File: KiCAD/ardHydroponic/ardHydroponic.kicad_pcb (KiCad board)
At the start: 2 copper layers, 7 parts, among them J1 3-pin_IRF5320_MOSFET_module_h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, J2 3-pin_IRF5320_MOSFET_module_h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, J3 3-pin_IRF5320_MOSFET_module_h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, J4 3-pin_IRF5320_MOSFET_module_h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, J5 4-pin_I2C_LCD_header, U1 DS18B20

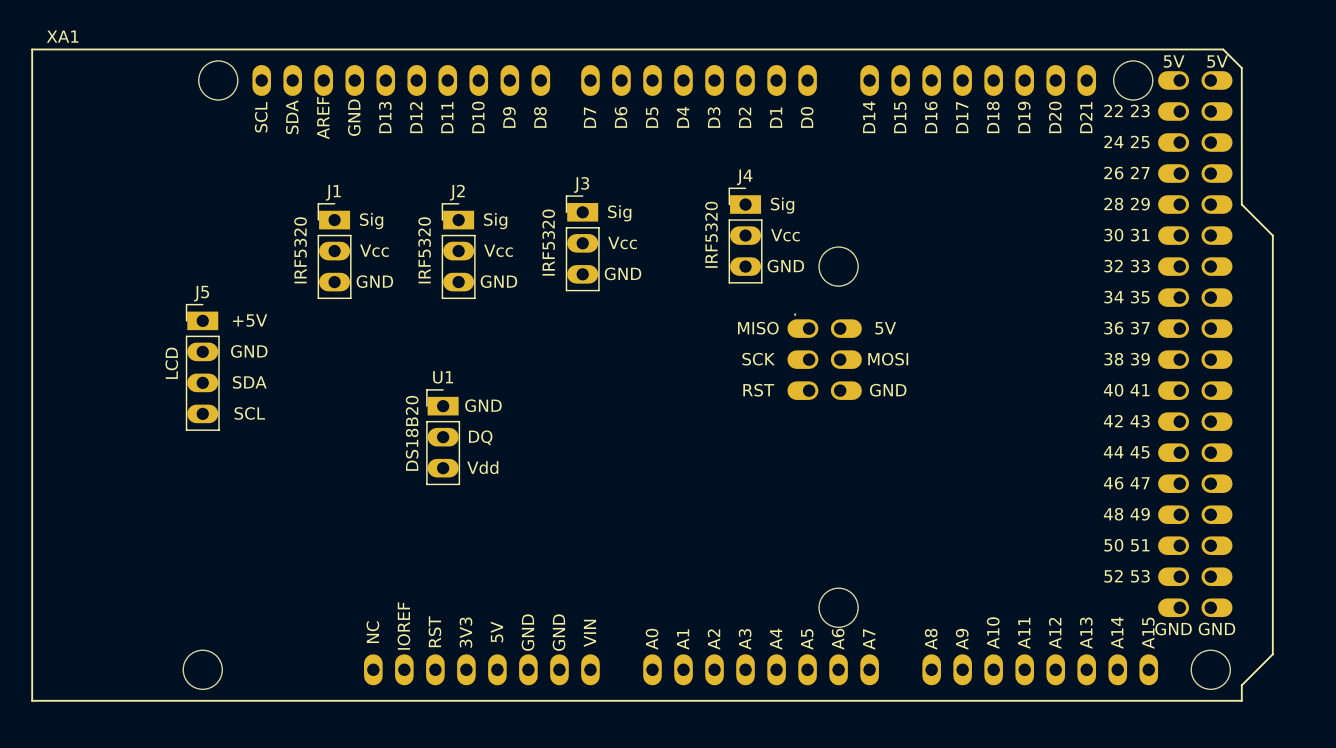
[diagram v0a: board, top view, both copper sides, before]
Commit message: new pins, schematics
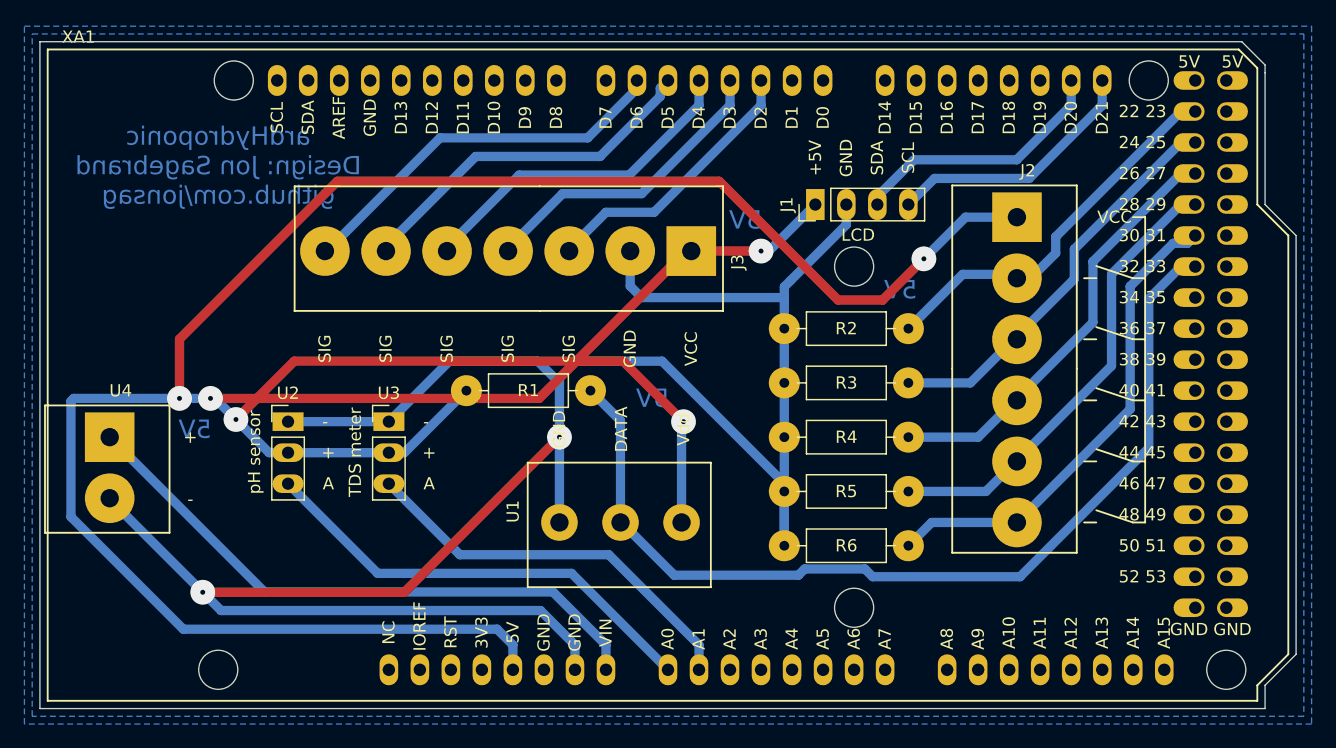
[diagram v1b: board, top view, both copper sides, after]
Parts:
- removed J4: 3-pin_IRF5320_MOSFET_module_header, My_Headers:3-pin_IRF5320_MOSFET_module_header_large
- removed J5: 4-pin_I2C_LCD_header, My_Headers:4-pin_I2C_LCD_header_larger
- added R1: 4.7k, My_Misc:R_Axial_DIN0207_L6.3mm_D2.5mm_P10.16mm_Horizontal_larger_pads, F.Cu at (134.6, 99.1)
- added R2: 10k, My_Misc:R_Axial_DIN0207_L6.3mm_D2.5mm_P10.16mm_Horizontal_larger_pads, F.Cu at (160.7, 94.0)
- added R3: 10k, My_Misc:R_Axial_DIN0207_L6.3mm_D2.5mm_P10.16mm_Horizontal_larger_pads, F.Cu at (160.7, 98.4)
- added R4: 10k, My_Misc:R_Axial_DIN0207_L6.3mm_D2.5mm_P10.16mm_Horizontal_larger_pads, F.Cu at (160.7, 102.9)
- added R5: 10k, My_Misc:R_Axial_DIN0207_L6.3mm_D2.5mm_P10.16mm_Horizontal_larger_pads, F.Cu at (160.7, 107.3)
- added R6: 10k, My_Misc:R_Axial_DIN0207_L6.3mm_D2.5mm_P10.16mm_Horizontal_larger_pads, F.Cu at (160.7, 111.8)
- added U2: pH sensor, My_Headers:3-pin_DFRobot_Gravity_pH-sensor_header_large, F.Cu at (120.0, 101.6)
- added U3: TDS meter, My_Headers:3-pin_DFRobot_Gravity_TDS-meter_header_large, F.Cu at (128.3, 101.6)
- added U4: Power in, My_Parts:2-pole_power_in_screw_terminal, F.Cu at (105.4, 102.9)
- J1: value 3-pin_IRF5320_MOSFET_module_header -> LCD display; footprint My_Headers:3-pin_IRF5320_MOSFET_module_header_large -> My_Headers:4-pin_I2C_LCD_header_larger
- J2: value 3-pin_IRF5320_MOSFET_module_header -> Buttons; footprint My_Headers:3-pin_IRF5320_MOSFET_module_header_large -> My_Parts:6-pole_5-NO_switch_screw_terminal
- J3: value 3-pin_IRF5320_MOSFET_module_header -> MOSFETs; footprint My_Headers:3-pin_IRF5320_MOSFET_module_header_large -> My_Parts:7-pole_6-MOSFET_screw_terminal
- U1: footprint My_Headers:3_pin_Dallas_1-wire_header_larger_pads -> My_Parts:3-pole_DS18B20_screw_terminal
- XA1: footprint My_Arduino:Arduino_Mega2560_Shield_large -> My_Arduino:Arduino_Mega2560_Shield__no_ICSP_large
- moved J2 45.7 mm to (179.7, 84.9)
- moved J1 39.4 mm to (163.2, 83.8), turned to 90 degrees
- moved U1 13.5 mm to (142.2, 109.9), turned to 90 degrees
- moved J3 9.44 mm to (153.0, 87.6), turned to 270 degrees
- moved XA1 1.27 mm to (100.3, 124.5)
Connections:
- J1 pad 1: Net-(J1-Pad1) -> +5V
- J1 pad 3: Net-(J1-Pad3) -> GND
- J2 pad 1: Net-(J2-Pad1) -> +5V
- J2 pad 2: Net-(J2-Pad2) -> button1
- J2 pad 3: Net-(J2-Pad3) -> button2
- J3 pad 1: Net-(J3-Pad1) -> +5V
- J3 pad 2: Net-(J3-Pad2) -> GND
- J3 pad 3: Net-(J3-Pad3) -> pH+
- U1 pad 1: Net-(U1-Pad1) -> GND
- U1 pad 2: Net-(U1-Pad2) -> dallas
- U1 pad 3: Net-(U1-Pad3) -> +5V
- XA1 pad 1: Net-(XA1-Pad1) -> nutrA
- XA1 pad 10: Net-(XA1-Pad10) -> +5V
- XA1 pad 100: Net-(XA1-Pad100) -> +6V
- XA1 pad 15: Net-(XA1-Pad15) -> stirrer
- XA1 pad 43: Net-(XA1-Pad43) -> Net-(J1-Pad7)
- XA1 pad 44: Net-(XA1-Pad44) -> Net-(J1-Pad5)
- XA1 pad 5: Net-(XA1-Pad5) -> nutrB
- XA1 pad 58: Net-(XA1-Pad58) -> dallas
- XA1 pad 6: Net-(XA1-Pad6) -> pH+
- XA1 pad 60: Net-(XA1-Pad60) -> button5
- XA1 pad 62: Net-(XA1-Pad62) -> GND
- XA1 pad 7: Net-(XA1-Pad7) -> pH-
- XA1 pad 72: Net-(XA1-Pad72) -> button4
- XA1 pad 74: Net-(XA1-Pad74) -> button3
- XA1 pad 76: Net-(XA1-Pad76) -> button2
- XA1 pad 78: Net-(XA1-Pad78) -> button1
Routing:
- net +5V: track 0.00 -> 284.9 mm, vias 0 -> 6
- net GND: track 0.00 -> 190.5 mm, vias 0 -> 2
- net dallas: track 0.00 -> 78.7 mm
- net +6V: track 0.00 -> 49.7 mm
- net button5: track 0.00 -> 39.9 mm
- net button4: track 0.00 -> 37.6 mm
- net Net-(U2-Pad3): track 0.00 -> 37.4 mm
- net button3: track 0.00 -> 35.4 mm
- net button2: track 0.00 -> 33.1 mm
- net Net-(U3-Pad3): track 0.00 -> 32.9 mm
- net stirrer: track 0.00 -> 32.5 mm
- net button1: track 0.00 -> 31.6 mm
- net nutrB: track 0.00 -> 29.7 mm
- net nutrA: track 0.00 -> 27.9 mm
- net pH-: track 0.00 -> 25.4 mm
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- added copper zone on B.Cu, net (none)
- added copper zone on B.Cu, net GND
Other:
- board outline added: 102.9 x 54.6 mm
- net class Default: clearance 0.2 -> 0.762; trace_width 0.25 -> 0.762; via_dia 0.8 -> 2.032
- rule trace_clearance: 0.2 -> 0.762
- board text added: "5V"
- board text added: "ardHydroponic Design: Jon Sagebrand github.com/jonsag"
